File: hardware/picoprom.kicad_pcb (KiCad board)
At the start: 2 copper layers, 81.8 x 53.3 mm, 15 parts, among them U1 Pico, U2 TXB0108PWR, U3 28C256

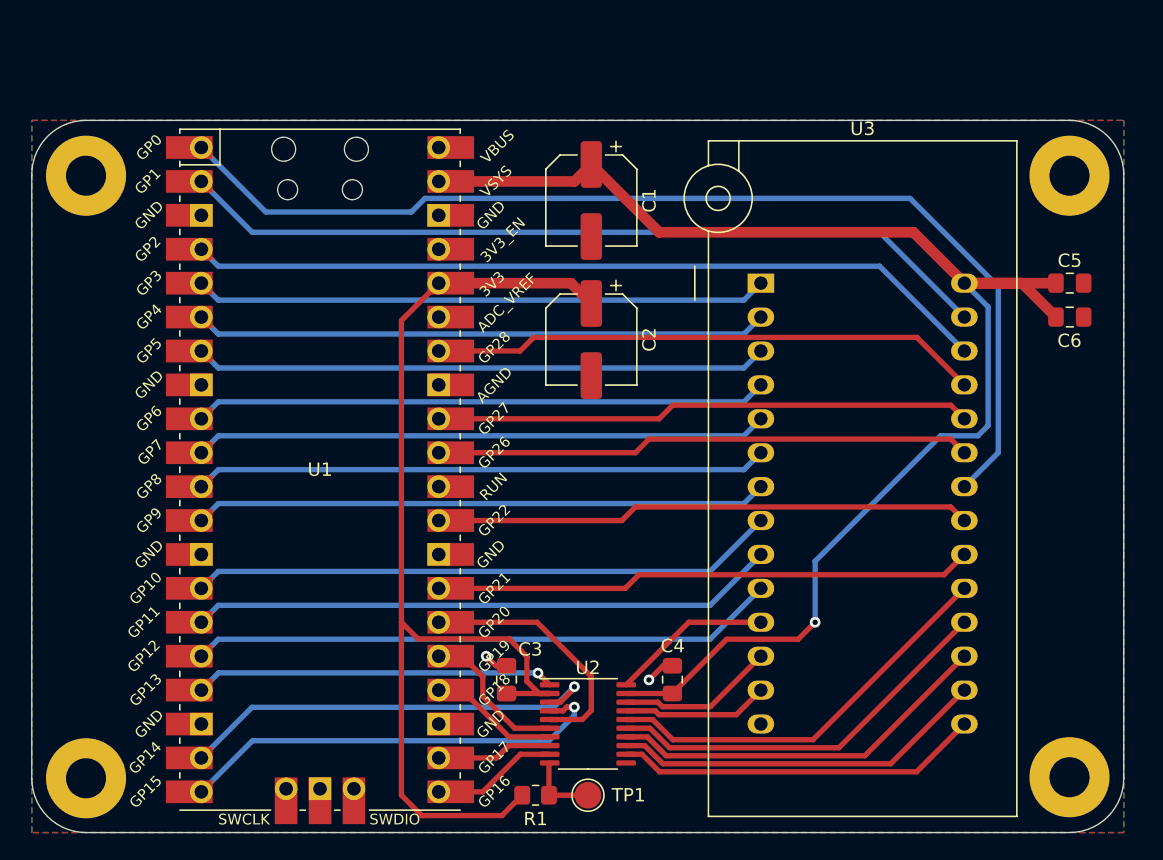
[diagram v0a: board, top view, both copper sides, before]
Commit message: Final edits to hardware for Rev0.
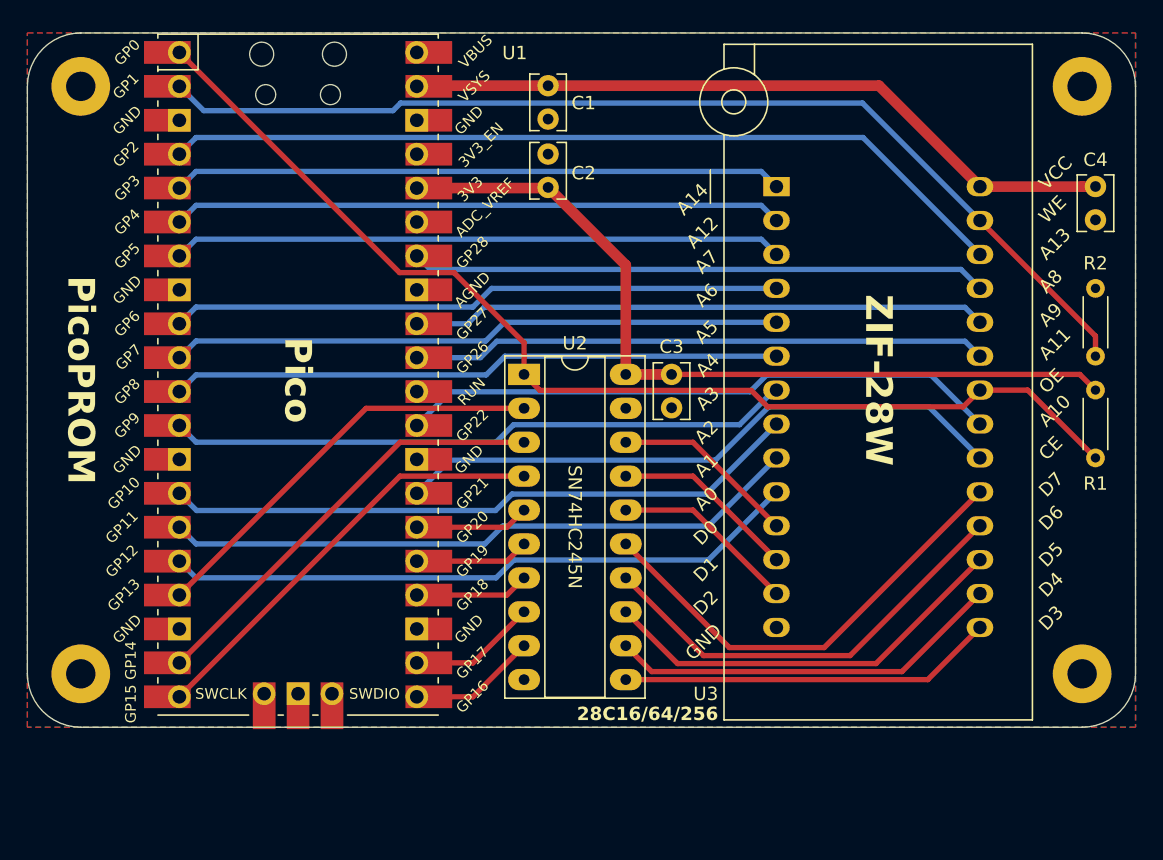
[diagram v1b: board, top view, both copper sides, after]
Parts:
- removed C5: 0.1u, Capacitor_SMD:C_0805_2012Metric_Pad1.18x1.45mm_HandSolder
- removed C6: 10u, Capacitor_SMD:C_0805_2012Metric_Pad1.18x1.45mm_HandSolder
- removed TP1: TXB_OE, TestPoint:TestPoint_Pad_D2.0mm
- added R2: 47k, Resistor_THT:R_Axial_DIN0204_L3.6mm_D1.6mm_P5.08mm_Horizontal, F.Cu at (180.0, 84.2)
- added REF**: OSHW-Logo2_9.8x8mm_SilkScreen, Symbol:OSHW-Logo2_9.8x8mm_SilkScreen, B.Cu at (163.8, 73.7)
- added REF**: WEEE-Logo_5.6x8mm_SilkScreen, Symbol:WEEE-Logo_5.6x8mm_SilkScreen, B.Cu at (163.8, 99.9)
- added REF**: QR-Code_12x12mm_SilkScreen, picoprom:QR-Code_12x12mm_SilkScreen, B.Cu at (120.3, 86.0)
- added REF**: KiCad-Logo2_5mm_SilkScreen, Symbol:KiCad-Logo2_5mm_SilkScreen, B.Cu at (163.8, 87.6)
- C1, C2: value 47u -> 0.1uF; footprint Capacitor_SMD:CP_Elec_6.3x5.8 -> Capacitor_THT:C_Rect_L4.0mm_W2.5mm_P2.50mm
- C3, C4: value 0.1u -> 0.1uF; footprint Capacitor_SMD:C_0805_2012Metric_Pad1.18x1.45mm_HandSolder -> Capacitor_THT:C_Rect_L4.0mm_W2.5mm_P2.50mm
- H1, H2, H3, H4: value 3mm -> M2; footprint MountingHole:MountingHole_3mm_Pad -> MountingHole:MountingHole_2.2mm_M2_Pad
- R1: footprint Resistor_SMD:R_0805_2012Metric_Pad1.20x1.40mm_HandSolder -> Resistor_THT:R_Axial_DIN0204_L3.6mm_D1.6mm_P5.08mm_Horizontal
- U2: value TXB0108PWR -> SN74HC245N; footprint Package_SO:TSSOP-20_4.4x6.5mm_P0.65mm -> Package_DIP:DIP-20_W7.62mm_Socket_LongPads
- moved R1 51.8 mm to (180.0, 86.8), turned to -90 degrees
- moved C4 48.7 mm to (180.0, 71.5), turned to -90 degrees
- moved U2 26.6 mm to (137.2, 85.6)
- moved C3 26.0 mm to (148.2, 85.6), turned to -90 degrees
- moved C2 11.8 mm to (139.0, 71.6), turned to 90 degrees
- moved C1 9.19 mm to (139.0, 64.0)
- moved H2 7.83 mm to (104.0, 108.0)
- moved H3 7.80 mm to (179.0, 108.0)
- moved U3 7.32 mm to (156.1, 71.5)
- moved U1 7.31 mm to (120.3, 85.6)
- moved H4 6.76 mm to (179.0, 64.0)
- moved H1 6.70 mm to (104.0, 64.0)
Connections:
- R1 pad 2: Net-(U2-OE) -> OE
- U2 pad 1: D0_3v3 -> OE
- U2 pad 10: Net-(U2-OE) -> GND
- U2 pad 11: GND -> D3_5v
- U2 pad 12: D3_5v -> D4_5v
- U2 pad 13: D4_5v -> D5_5v
- U2 pad 14: D5_5v -> D6_5v
- U2 pad 15: D6_5v -> D7_5v
- U2 pad 16: D7_5v -> D2_5v
- U2 pad 17: D2_5v -> D1_5v
- U2 pad 18: D1_5v -> D0_5v
- U2 pad 19: +5V -> GND
- U2 pad 2: +3V3 -> D0_3v3
- U2 pad 20: D0_5v -> +3V3
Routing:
- net +5V: track 107.9 -> 54.0 mm, vias 1 -> 0
- net +3V3: track 79.5 -> 61.9 mm
- net WE: track 61.4 -> 78.4 mm
- net D7_3v3: track 19.1 -> 8.57 mm
- net CE: track 40.4 -> 46.5 mm
- net Net-(U2-OE): track 5.37 -> 0.00 mm
- net A10: track 40.2 -> 45.3 mm
- net D0_3v3: track 27.0 -> 31.6 mm, vias 1 -> 0
- net GND: track 4.02 -> 0.00 mm, vias 2 -> 0
- net A2: track 44.0 -> 47.9 mm
- net D7_5v: track 30.7 -> 34.6 mm
- net A3: track 43.0 -> 46.9 mm
- net A1: track 44.0 -> 47.9 mm
- net A0: track 44.0 -> 47.9 mm
- net A13: track 60.3 -> 64.1 mm
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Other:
- board size 81.8 x 53.3 mm -> 83 x 52 mm
- board text added: "28C16/64/256"
- board text added: "A0"
- board text added: "A1"
- board text added: "A10"
- board text added: "A11"
- board text added: "A12"
- board text added: "A13"
- board text added: "A14"
- board text added: "A2"
- board text added: "A3"
- board text added: "A4"
- board text added: "A5"
- board text added: "A6"
- board text added: "A7"
- board text added: "A8"
- board text added: "A9"
- board text added: "CE"
- board text added: "D0"
- board text added: "D1"
- board text added: "D2"
- board text added: "D3"
- board text added: "D4"
- board text added: "D5"
- board text added: "D6"
- board text added: "D7"
- board text added: "GND"
- board text added: "Hardware by Cooper Dalrymple Firmware by George Foot 2024-02-19 Rev0"
- board text added: "OE"
- board text added: "Pico"
- board text added: "PicoPROM"
- board text added: "SN74HC245N"
- board text added: "VCC"
- board text added: "WE"
- board text added: "ZIF-28W"
